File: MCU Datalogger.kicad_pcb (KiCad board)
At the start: 2 copper layers, 52.1 x 33 mm, 29 parts, among them J1 Conn_01x04_Pin, J2 Conn_01x09_Pin, J3 Conn_01x04_Pin, J4 Conn_02x03_Odd_Even, U1 DS1337S+, U2 24LC1025, U3 24LC1025, U4 ATMEGA328P-AU, Y1 32.768 KHz, Y2 16 MHz

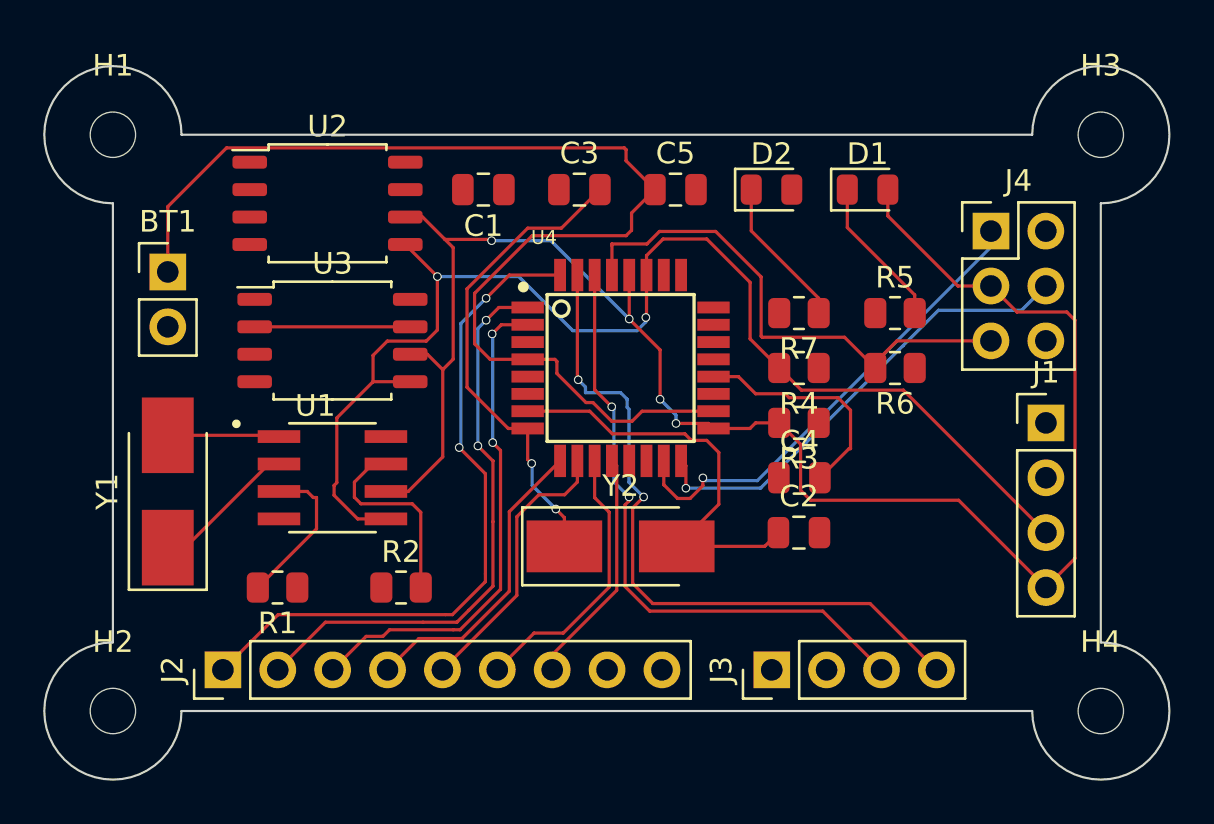
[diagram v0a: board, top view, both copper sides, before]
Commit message: Completed wiring. Many improvements pending.
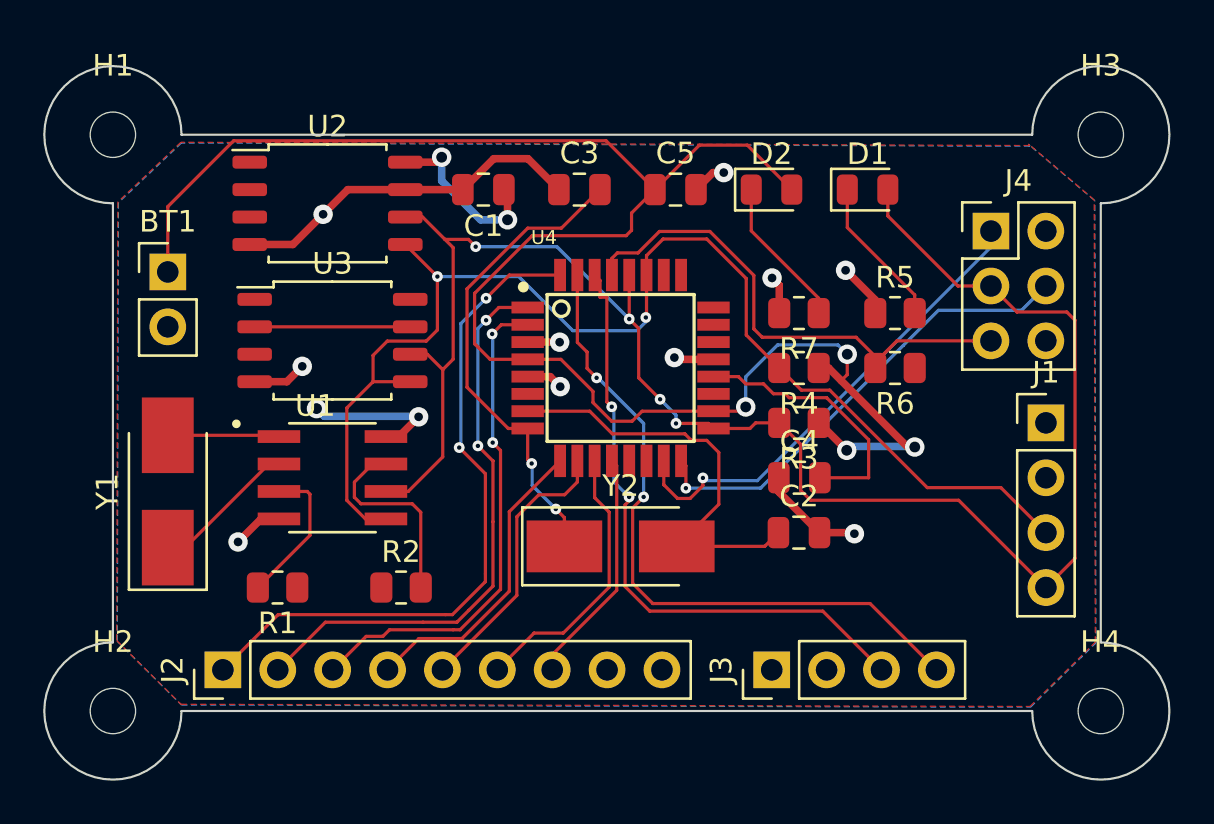
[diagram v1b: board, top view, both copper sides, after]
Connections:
- BT1 pad 1: Net-(BT1-+) -> /Vcc
- C5 pad 1: Net-(BT1-+) -> /Vcc
- D2 pad 2: Net-(BT1-+) -> /Vcc
- U4 pad 18: Net-(BT1-+) -> /Vcc
- U4 pad 4: Net-(BT1-+) -> /Vcc
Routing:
- net /Vcc: track 0.00 -> 97.7 mm, vias 0 -> 8
- net Net-(BT1-+): track 54.0 -> 0.00 mm
- net GND: track 0.00 -> 37.7 mm, vias 0 -> 10
- net Net-(U4-AREF): track 10.8 -> 12.5 mm
- net /TX: track 32.4 -> 31.5 mm
- net /SDA: track 59.7 -> 59.0 mm
- added copper zone on F.Cu, net /Vcc
- added copper zone on B.Cu, net GND
